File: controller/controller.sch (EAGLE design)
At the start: 26 parts, among them IC1 ATtiny25, IC2 74HC595N

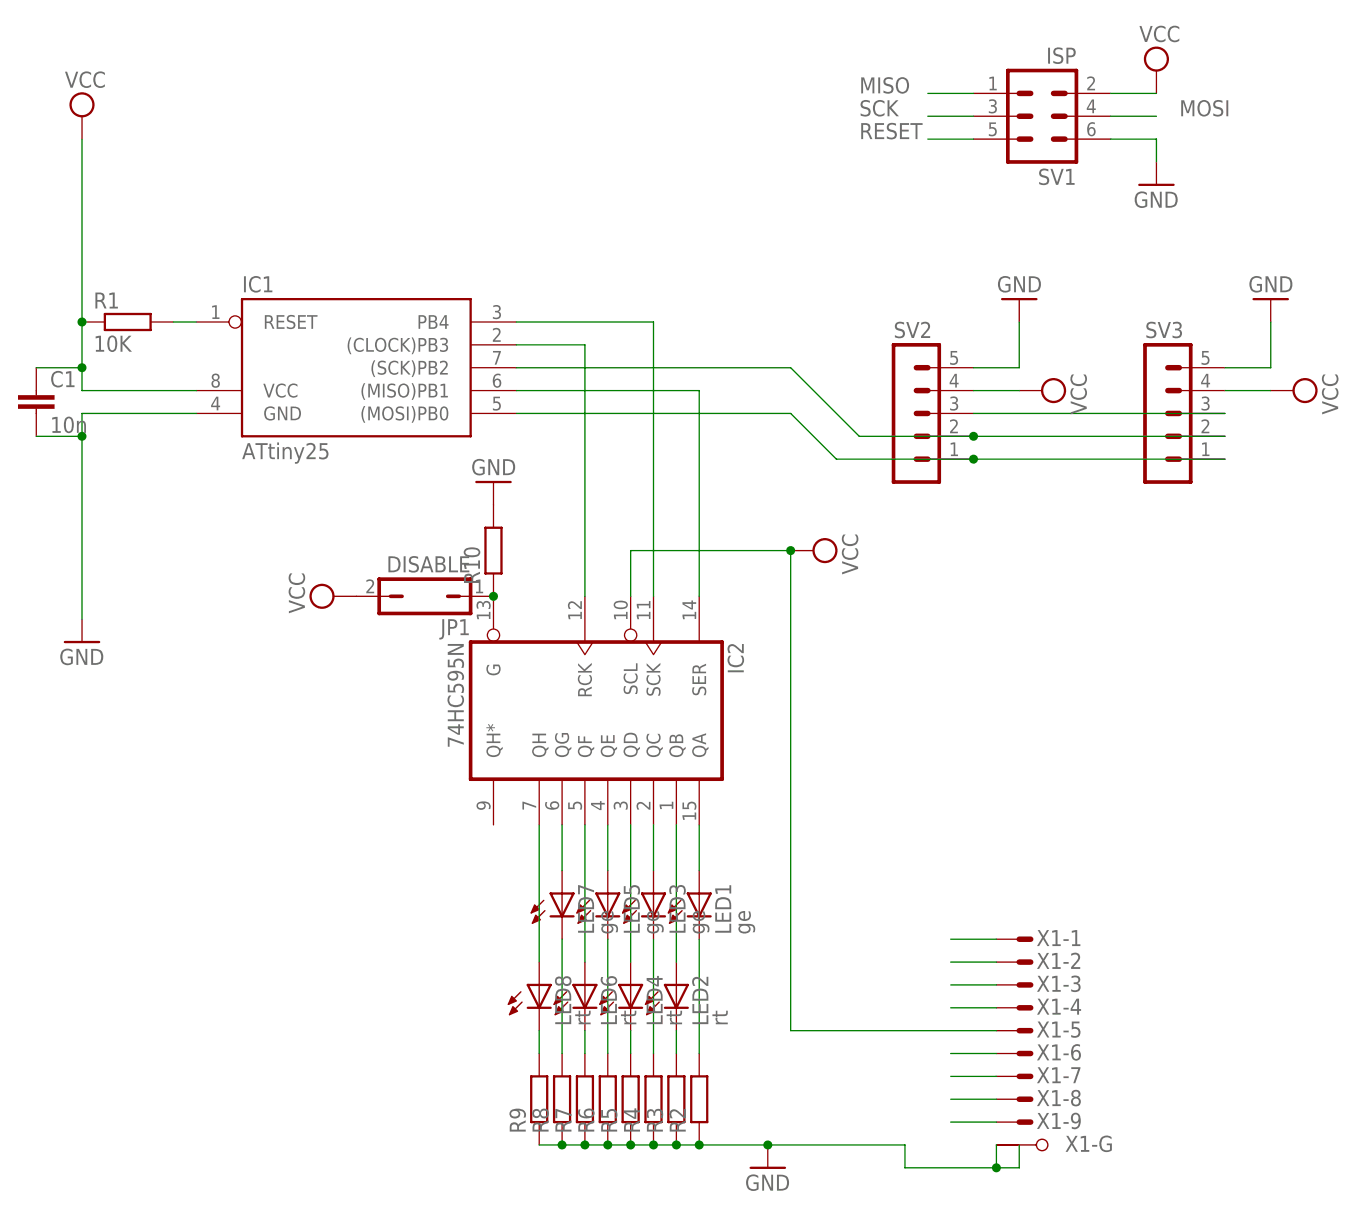
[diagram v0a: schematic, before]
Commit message: Routing erster Versuch
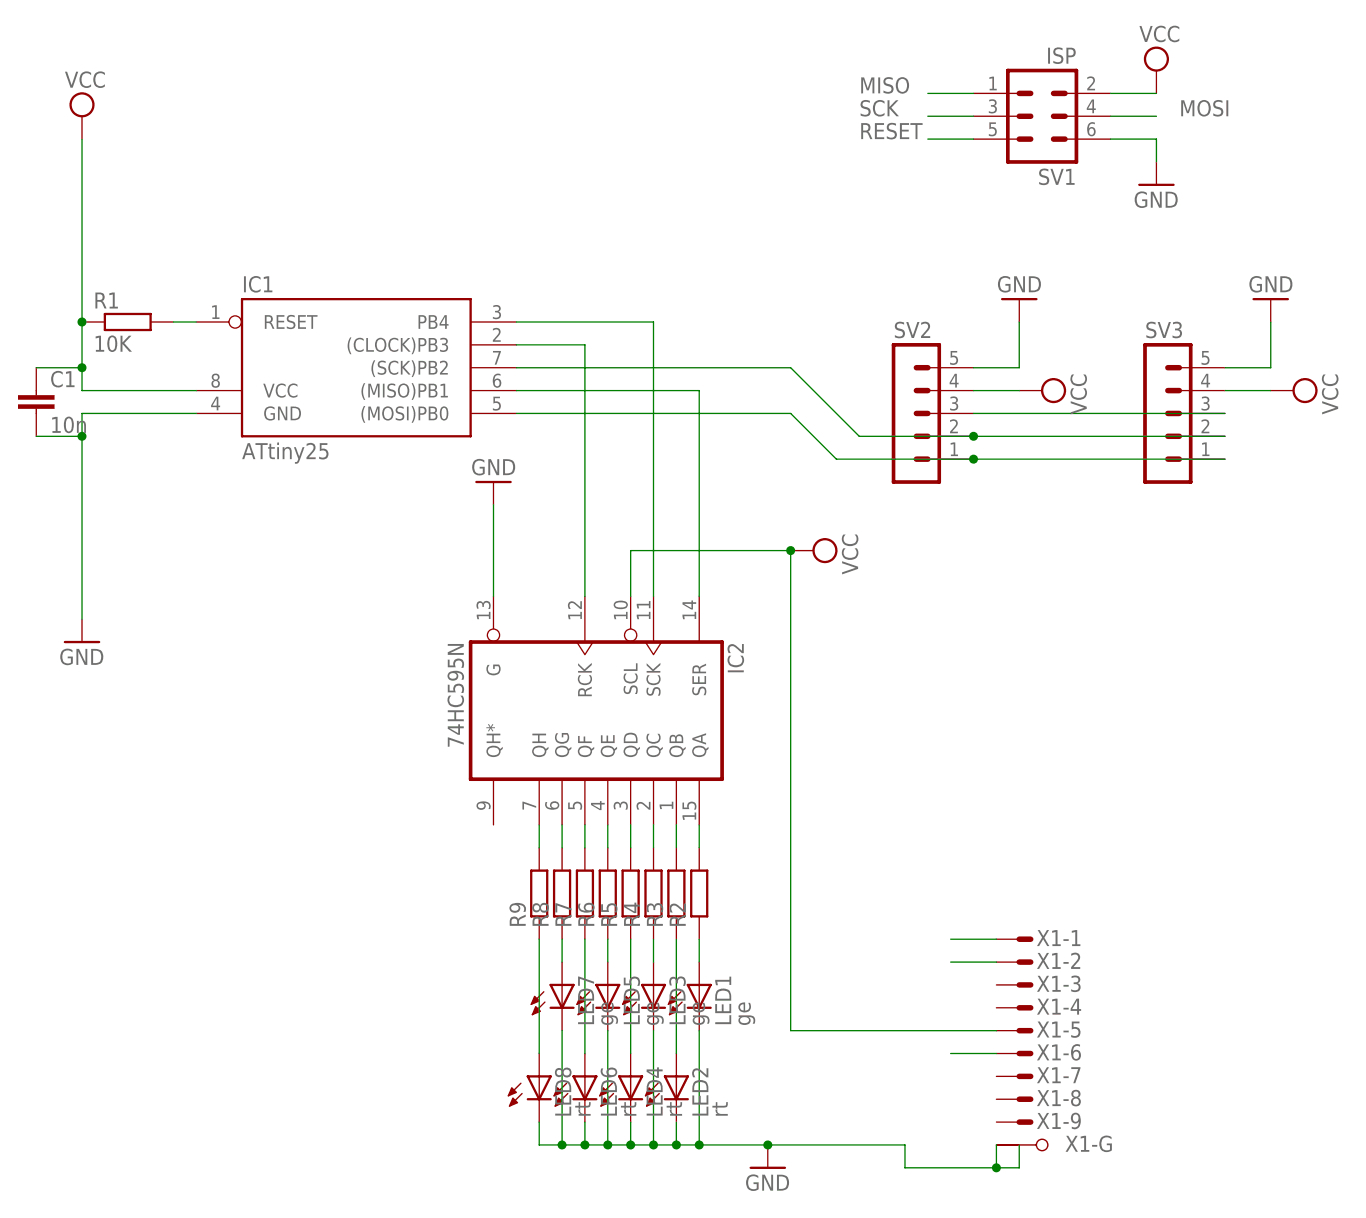
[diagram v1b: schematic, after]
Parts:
- removed JP1: DISABLE, jumper:JP1Q
- removed R10: (no value), resistor:R-EU_0617/5V
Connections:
- removed net N$13: LED6.C, R7.2
- removed net N$14: LED5.C, R6.2
- removed net N$16: LED8.C, R9.2
- removed net N$17: LED7.C, R8.2
- removed net N$4: IC2A.G, JP1.1, R10.1
- new net N$11: LED7.A, R8.1
- new net N$12: LED8.A, R9.1
- new net N$5: LED1.A, R2.1
- new net N$8: LED4.A, R5.1
- net GND: now also IC2A.G, LED1.C, LED2.C, LED3.C, LED4.C, LED5.C, LED6.C, LED7.C, LED8.C; no longer R10.2, R2.1, R3.1, R4.1, R5.1, R6.1, R7.1, R8.1, R9.1
- net N$10: now also LED6.A, R7.1; no longer LED3.C, R4.2
- net N$6: now also LED2.A, R3.1; no longer LED2.C, R3.2
- net N$7: now also LED3.A, R4.1; no longer LED1.C, R2.2
- net N$9: now also LED5.A, R6.1; no longer LED4.C, R5.2
- net QA: now also R2.2; no longer LED1.A
- net QB: now also R3.2, X1-6.M; no longer LED2.A, X1-2.M
- net QC: now also R4.2, X1-2.M; no longer LED3.A, X1-3.M
- net QD: now also R5.2; no longer LED4.A, X1-4.M
- net QE: now also R6.2; no longer LED5.A, X1-6.M
- net QF: now also R7.2; no longer LED6.A, X1-7.M
- net QG: now also R8.2; no longer LED7.A, X1-8.M
- net QH: now also R9.2; no longer LED8.A, X1-9.M
- net VCC: no longer JP1.2
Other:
- moved on the sheet: LED1, LED2, LED3, LED4, LED5, LED6, LED7, LED8, R2, R3, R4, R5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
